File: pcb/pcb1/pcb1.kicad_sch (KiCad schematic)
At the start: 1 part, among them U1 ESP32-DevKitC

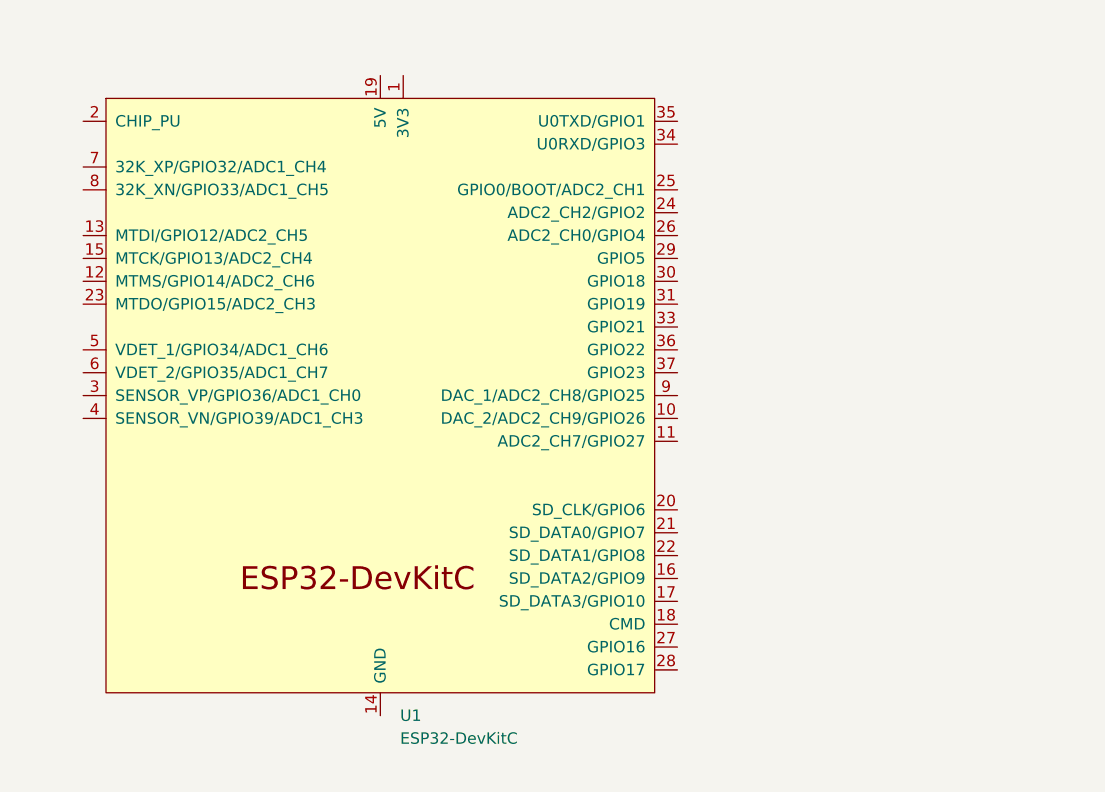
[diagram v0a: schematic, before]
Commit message: pcb2
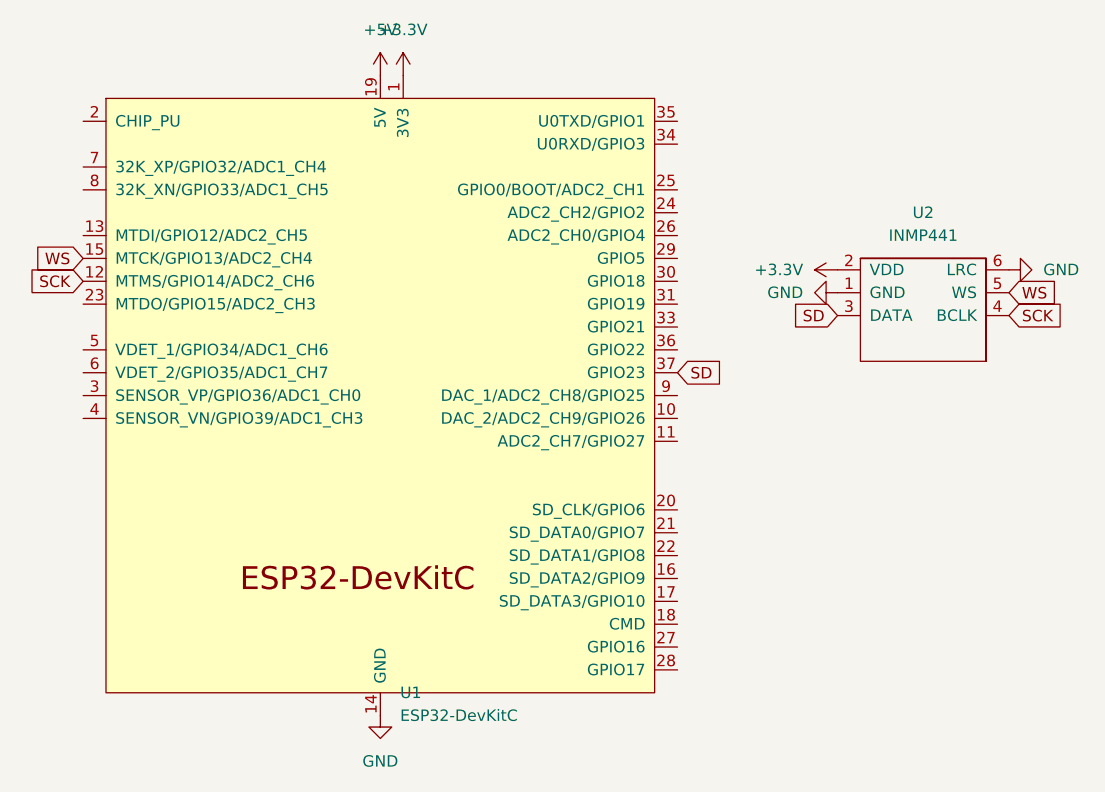
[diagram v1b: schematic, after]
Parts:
- added U2: INMP441, symbol INMP441:INMP441
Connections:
- net +3.3V: now reaches U1.1 (3V3)
- net +3.3V: now also U2.2 (VDD)
- net SCK: now reaches U1.12 (MTMS/GPIO14/ADC2_CH6)
- net SCK: now also U2.4 (BCLK)
- net GND: now reaches U1.14 (GND), U1.32 (GND), U1.38 (GND)
- net GND: now also U2.1 (GND), U2.6 (LRC)
- net WS: now reaches U1.15 (MTCK/GPIO13/ADC2_CH4)
- net WS: now also U2.5 (WS)
- net +5V: now reaches U1.19 (5V)
- net SD: now reaches U1.37 (GPIO23)
- net SD: now also U2.3 (DATA)
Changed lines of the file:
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@@
 (kicad_sch (version 20230121) (generator eeschema)
   (paper "A4")
+  (global_label "WS" (shape input) (at 69.85 60.96 180) (fields_autoplaced)
+    (effects (font (size 1.27 1.27)) (justify right))
+    (property "Intersheetrefs" "${INTERSHEET_REFS}" (at 64.2039 60.96 0)
+      (effects (font (size 1.27 1.27)) (justify right) hide)
+    )
+  )
+  (global_label "SD" (shape input) (at 135.89 73.66 0) (fields_autoplaced)
+    (effects (font (size 1.27 1.27)) (justify left))
+    (property "Intersheetrefs" "${INTERSHEET_REFS}" (at 141.3547 73.66 0)
+      (effects (font (size 1.27 1.27)) (justify left) hide)
+    )
+  )
+  (global_label "WS" (shape input) (at 172.72 64.77 0) (fields_autoplaced)
+    (effects (font (size 1.27 1.27)) (justify left))
+    (property "Intersheetrefs" "${INTERSHEET_REFS}" (at 178.3661 64.77 0)
+      (effects (font (size 1.27 1.27)) (justify left) hide)
+    )
+  )
+  (global_label "SD" (shape input) (at 153.67 67.31 180) (fields_autoplaced)
+    (effects (font (size 1.27 1.27)) (justify right))
+    (property "Intersheetrefs" "${INTERSHEET_REFS}" (at 148.2053 67.31 0)
+      (effects (font (size 1.27 1.27)) (justify right) hide)
+    )
+  )
+  (global_label "SCK" (shape input) (at 69.85 63.5 180) (fields_autoplaced)
+    (effects (font (size 1.27 1.27)) (justify right))
+    (property "Intersheetrefs" "${INTERSHEET_REFS}" (at 63.1153 63.5 0)
+      (effects (font (size 1.27 1.27)) (justify right) hide)
+    )
+  )
+  (global_label "SCK" (shape input) (at 172.72 67.31 0) (fields_autoplaced)
+    (effects (font (size 1.27 1.27)) (justify left))
+    (property "Intersheetrefs" "${INTERSHEET_REFS}" (at 179.4547 67.31 0)
+      (effects (font (size 1.27 1.27)) (justify left) hide)
+    )
+  )
+  (symbol (lib_id "power:GND") (at 102.87 111.76 0) (unit 1)
+    (in_bom yes) (on_board yes) (dnp no) (fields_autoplaced)
+    (property "Reference" "#PWR03" (at 102.87 118.11 0)
+      (effects (font (size 1.27 1.27)) hide)
+    )
+    (property "Value" "GND" (at 102.87 116.84 0)
+      (effects (font (size 1.27 1.27)))
+    )
+    (property "Footprint" "" (at 102.87 111.76 0)
+      (effects (font (size 1.27 1.27)) hide)
+    )
+    (property "Datasheet" "" (at 102.87 111.76 0)
+      (effects (font (size 1.27 1.27)) hide)
+    )
+    (pin "1")
+    (instances
+      (project "pcb1"
+        (path "/5b656699-2e5a-40bb-9ba1-72287c2297ae"
+          (reference "#PWR03") (unit 1)
+        )
+      )
+    )
+  )
+  (symbol (lib_id "power:+3.3V") (at 153.67 62.23 90) (unit 1)
+    (in_bom yes) (on_board yes) (dnp no) (fields_autoplaced)
+    (property "Reference" "#PWR05" (at 157.48 62.23 0)
+      (effects (font (size 1.27 1.27)) hide)
+    )
+    (property "Value" "+3.3V" (at 149.86 62.23 90)
+      (effects (font (size 1.27 1.27)) (justify left))
+    )
+    (property "Footprint" "" (at 153.67 62.23 0)
+      (effects (font (size 1.27 1.27)) hide)
+    )
+    (property "Datasheet" "" (at 153.67 62.23 0)
+      (effects (font (size 1.27 1.27)) hide)
+    )
+    (pin "1")
+    (instances
+      (project "pcb1"
+        (path "/5b656699-2e5a-40bb-9ba1-72287c2297ae"
+          (reference "#PWR05") (unit 1)
+        )
+      )
+    )
+  )
+  (symbol (lib_id "power:GND") (at 172.72 62.23 90) (unit 1)
+    (in_bom yes) (on_board yes) (dnp no) (fields_autoplaced)
+    (property "Reference" "#PWR06" (at 179.07 62.23 0)
+      (effects (font (size 1.27 1.27)) hide)
+    )
+    (property "Value" "GND" (at 176.53 62.23 90)
+      (effects (font (size 1.27 1.27)) (justify right))
+    )
+    (property "Footprint" "" (at 172.72 62.23 0)
+      (effects (font (size 1.27 1.27)) hide)
+    )
+    (property "Datasheet" "" (at 172.72 62.23 0)
+      (effects (font (size 1.27 1.27)) hide)
+    )
+    (pin "1")
+    (instances
+      (project "pcb1"
+        (path "/5b656699-2e5a-40bb-9ba1-72287c2297ae"
+          (reference "#PWR06") (unit 1)
+        )
+      )
+    )
+  )
+  (symbol (lib_id "power:GND") (at 153.67 64.77 270) (unit 1)
+    (in_bom yes) (on_board yes) (dnp no) (fields_autoplaced)
+    (property "Reference" "#PWR04" (at 147.32 64.77 0)
+      (effects (font (size 1.27 1.27)) hide)
+    )
+    (property "Value" "GND" (at 149.86 64.77 90)
+      (effects (font (size 1.27 1.27)) (justify right))
+    )
+    (property "Footprint" "" (at 153.67 64.77 0)
+      (effects (font (size 1.27 1.27)) hide)
+    )
+    (property "Datasheet" "" (at 153.67 64.77 0)
+      (effects (font (size 1.27 1.27)) hide)
+    )
+    (pin "1")
+    (instances
+      (project "pcb1"
+        (path "/5b656699-2e5a-40bb-9ba1-72287c2297ae"
+          (reference "#PWR04") (unit 1)
+        )
+      )
+    )
+  )
+  (symbol (lib_id "power:+5V") (at 102.87 40.64 0) (unit 1)
+    (in_bom yes) (on_board yes) (dnp no) (fields_autoplaced)
+    (property "Reference" "#PWR02" (at 102.87 44.45 0)
+      (effects (font (size 1.27 1.27)) hide)
+    )
+    (property "Value" "+5V" (at 102.87 35.56 0)
+      (effects (font (size 1.27 1.27)))
+    )
+    (property "Footprint" "" (at 102.87 40.64 0)
+      (effects (font (size 1.27 1.27)) hide)
+    )
+    (property "Datasheet" "" (at 102.87 40.64 0)
+      (effects (font (size 1.27 1.27)) hide)
+    )
+    (pin "1")
+    (instances
+      (project "pcb1"
+        (path "/5b656699-2e5a-40bb-9ba1-72287c2297ae"
+          (reference "#PWR02") (unit 1)
+        )
+      )
+    )
+  )
   (symbol (lib_id "PCM_Espressif:ESP32-DevKitC") (at 102.87 76.2 0) (unit 1)
-    (in_bom yes) (on_board yes) (dnp no) (fields_autoplaced)
-    (property "Reference" "U1" (at 105.0641 111.76 0)
+    (in_bom yes) (on_board yes) (dnp no)
+    (property "Reference" "U1" (at 105.0641 109.22 0)
       (effects (font (size 1.27 1.27)) (justify left))
     )
-    (property "Value" "ESP32-DevKitC" (at 105.0641 114.3 0)
+    (property "Value" "ESP32-DevKitC" (at 105.0641 111.76 0)
       (effects (font (size 1.27 1.27)) (justify left))
     )
@@
         )
       )
+    )
+  )
+  (symbol (lib_id "INMP441:INMP441") (at 163.83 58.42 0) (unit 1)
+    (in_bom yes) (on_board yes) (dnp no) (fields_autoplaced)
+    (property "Reference" "U2" (at 163.195 55.88 0)
+      (effects (font (size 1.27 1.27)))
+    )
+    (property "Value" "INMP441" (at 163.195 58.42 0)
+      (effects (font (size 1.27 1.27)))
+    )
+    (property "Footprint" "" (at 163.83 58.42 0)
+      (effects (font (size 1.27 1.27)) hide)
+    )
+    (property "Datasheet" "" (at 163.83 58.42 0)
+      (effects (font (size 1.27 1.27)) hide)
+    )
+    (pin "6")
+    (pin "1")
+    (pin "2")
+    (pin "4")
+    (pin "5")
+    (pin "3")
+    (instances
+      (project "pcb1"
+        (path "/5b656699-2e5a-40bb-9ba1-72287c2297ae"
+          (reference "U2") (unit 1)
+        )
+      )
+    )
+  )
+  (symbol (lib_id "power:+3.3V") (at 105.41 40.64 0) (unit 1)
+    (in_bom yes) (on_board yes) (dnp no) (fields_autoplaced)
+    (property "Reference" "#PWR01" (at 105.41 44.45 0)
+      (effects (font (size 1.27 1.27)) hide)
+    )
+    (property "Value" "+3.3V" (at 105.41 35.56 0)
+      (effects (font (size 1.27 1.27)))
+    )
+    (property "Footprint" "" (at 105.41 40.64 0)
+      (effects (font (size 1.27 1.27)) hide)
+    )
+    (property "Datasheet" "" (at 105.41 40.64 0)
+      (effects (font (size 1.27 1.27)) hide)
+    )
+    (pin "1")
+    (instances
+      (project "pcb1"
+        (path "/5b656699-2e5a-40bb-9ba1-72287c2297ae"
+          (reference "#PWR01") (unit 1)
+        )
+      )

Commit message: github2
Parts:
- U2: footprint (none) -> inmp441:INMP441
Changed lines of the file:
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@@
       (effects (font (size 1.27 1.27)))
     )
-    (property "Footprint" "" (at 163.83 58.42 0)
+    (property "Footprint" "inmp441:INMP441" (at 163.83 58.42 0)
       (effects (font (size 1.27 1.27)) hide)
     )
